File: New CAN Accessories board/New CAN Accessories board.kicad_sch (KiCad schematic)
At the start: 85 parts, among them J1 39301040, J10 39301040, J11 ATF13-2P-BM03, J2 39301040, J3 39301040, J4 39301040, J5 39301040, J6 39301040, J7 39301040, J8 39301040, J9 39301060, Q1 IRLML6344TRPBF, Q2 IRLML6344TRPBF, Q3 IRLML6344TRPBF, Q4 IRLML6344TRPBF, Q5 IRLML6344TRPBF, Q6 IRLML6344TRPBF, Q7 IRLML6344TRPBF, Q8 IRLML6344TRPBF, T1 MCP2562FD-E_SN, U1 NUCLEO_L432KC

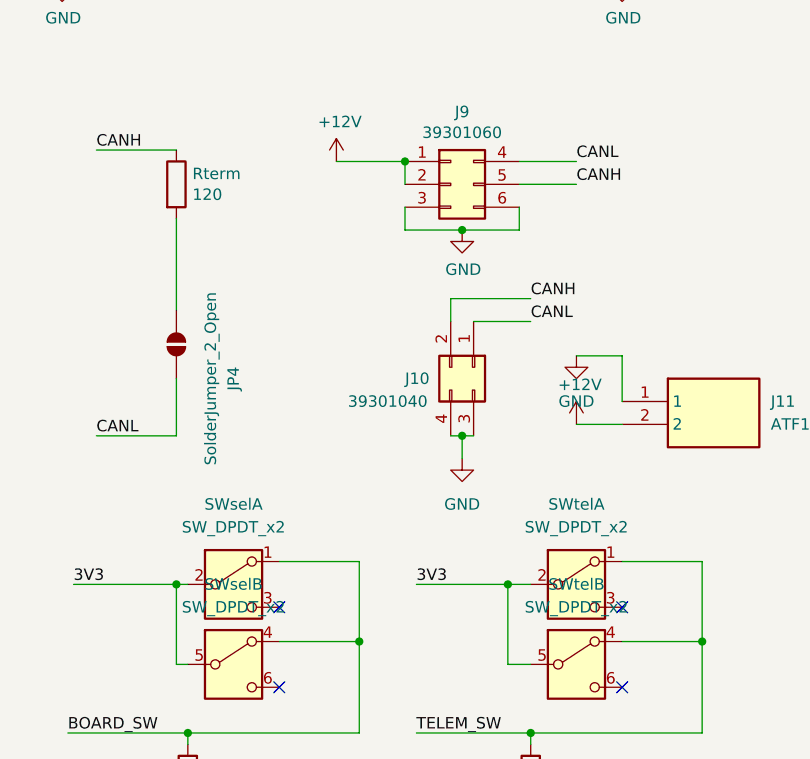
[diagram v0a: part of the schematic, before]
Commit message: Annotate
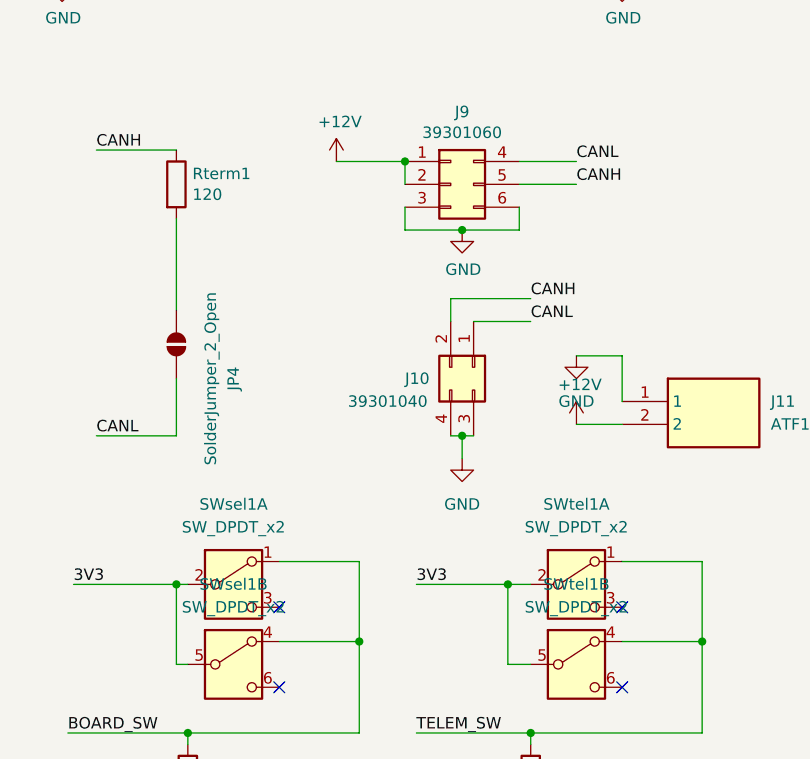
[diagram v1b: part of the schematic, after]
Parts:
- renumbered Rterm to Rterm1, SWsel to SWsel1, SWtel to SWtel1
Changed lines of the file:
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@@
 		(on_board yes)
 		(dnp no)
-		(property "Reference" "Rterm"
+		(property "Reference" "Rterm1"
 			(at 44.958 144.8816 0)
 			(effects
@@
 			(project "New CAN Accessories board"
 				(path "/88340f43-3f46-45a6-9393-130e00dc3071"
-					(reference "Rterm")
+					(reference "Rterm1")
 					(unit 1)
 				)
@@
 		(dnp no)
 		(fields_autoplaced yes)
-		(property "Reference" "SWsel"
+		(property "Reference" "SWsel1"
 			(at 49.53 190.5 0)
 			(effects
@@
 			(project "New CAN Accessories board"
 				(path "/88340f43-3f46-45a6-9393-130e00dc3071"
-					(reference "SWsel")
+					(reference "SWsel1")
 					(unit 2)
 				)
@@
 		(dnp no)
 		(fields_autoplaced yes)
-		(property "Reference" "SWsel"
+		(property "Reference" "SWsel1"
 			(at 49.53 181.61 0)
 			(effects
@@
 			(project ""
 				(path "/88340f43-3f46-45a6-9393-130e00dc3071"
-					(reference "SWsel")
+					(reference "SWsel1")
 					(unit 1)
 				)
@@
 		(dnp no)
 		(fields_autoplaced yes)
-		(property "Reference" "SWtel"
+		(property "Reference" "SWtel1"
 			(at 87.63 190.5 0)
 			(effects
@@
 			(project "New CAN Accessories board"
 				(path "/88340f43-3f46-45a6-9393-130e00dc3071"
-					(reference "SWtel")
+					(reference "SWtel1")
 					(unit 2)
 				)
@@
 		(dnp no)
 		(fields_autoplaced yes)
-		(property "Reference" "SWtel"
+		(property "Reference" "SWtel1"
 			(at 87.63 181.61 0)
 			(effects
@@
 			(project "New CAN Accessories board"
 				(path "/88340f43-3f46-45a6-9393-130e00dc3071"
-					(reference "SWtel")
+					(reference "SWtel1")
 					(unit 1)
 				)
